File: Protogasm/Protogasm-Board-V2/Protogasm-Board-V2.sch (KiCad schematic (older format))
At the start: 8 parts

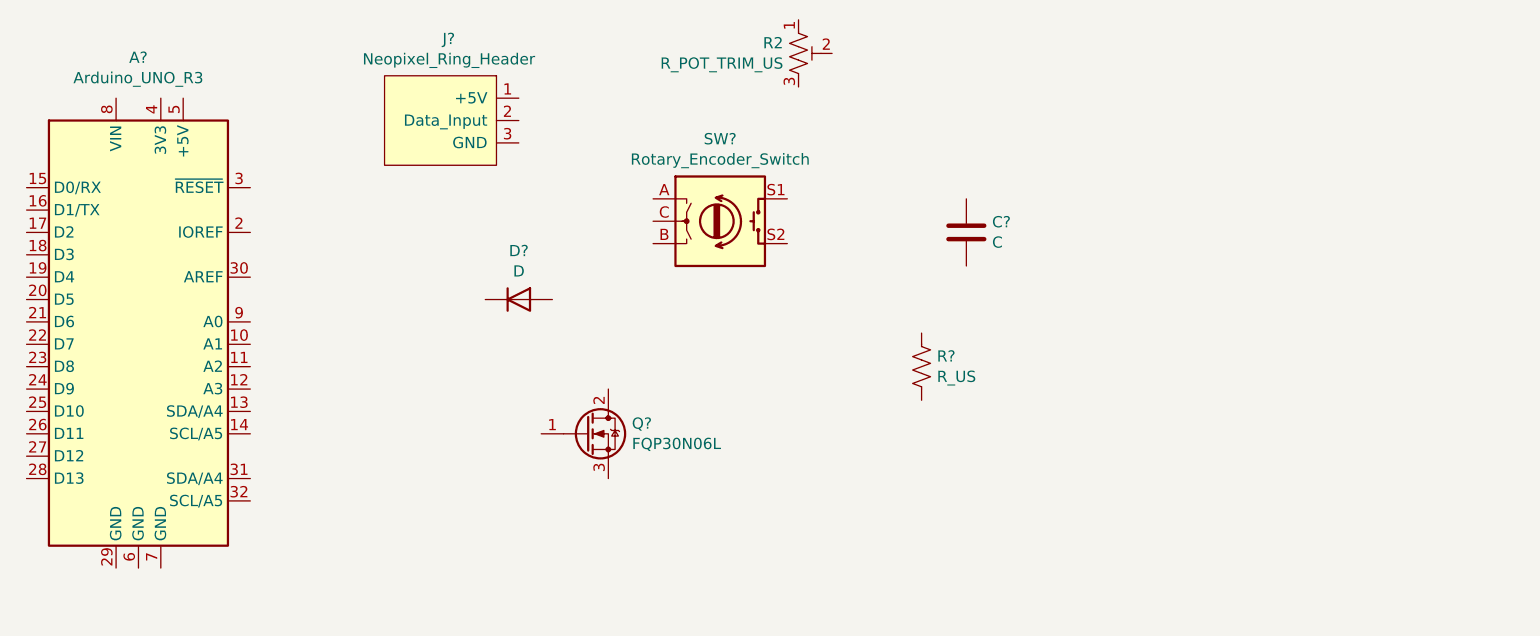
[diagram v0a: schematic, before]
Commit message: Complete the schematic
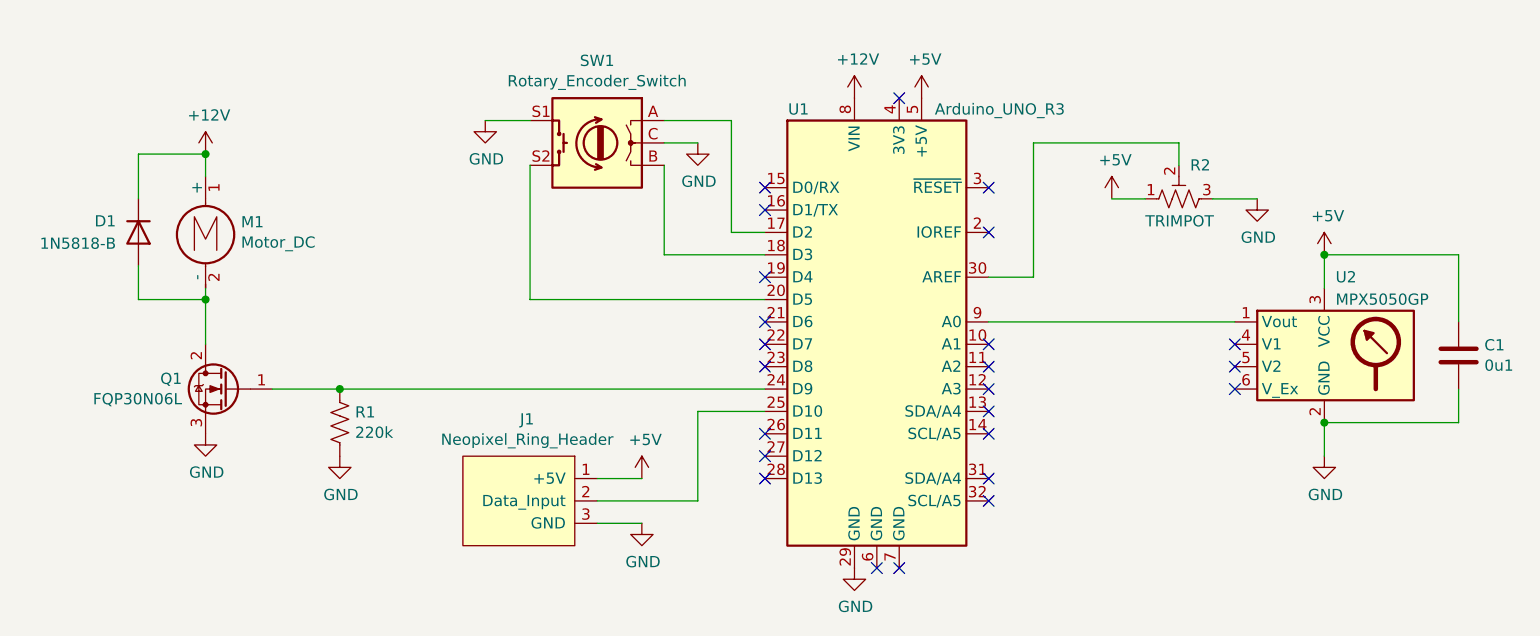
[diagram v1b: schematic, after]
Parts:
- added M1: Motor_DC, symbol Motor:Motor_DC
- added U2: MPX5050GP, symbol custom-symbols:MPX5050GP
- C1: renamed from C?; value C -> 0u1
- D1: renamed from D?; value D -> 1N5818-B
- R1: renamed from R?; value R_US -> 220k
- R2: value R_POT_TRIM_US -> TRIMPOT
- gave numbers to parts that had none: 4
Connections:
- net at U1.17 (D2): now also SW1.A
- net at U1.18 (D3): now also SW1.B
- net at U1.20 (D5): now also SW1.S2
- net at U1.24 (D9): now also Q1.1 (G), R1.1
- net at U1.25 (D10): now also J1.2 (Data_Input)
- net GND: now reaches U1.29 (GND)
- net GND: now also C1.2, J1.3 (GND), Q1.3 (S), R1.2, R2.3, SW1.C, SW1.S1, U2.2 (GND)
- net at U1.30 (AREF): now also R2.2
- net +5V: now reaches U1.5 (+5V)
- net +5V: now also C1.1, J1.1 (+5V), R2.1, U2.3 (VCC)
- net +12V: now reaches U1.8 (VIN)
- net +12V: now also D1.1 (K), M1.1 (+)
- net at U1.9 (A0): now also U2.1 (Vout)
- net at D1.2 (A): now also Q1.2 (D), M1.2 (-)
- no-connect marks 0 -> 24
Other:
- moved on the sheet: C1, D1, J1, Q1, R1, R2, SW1, U1
